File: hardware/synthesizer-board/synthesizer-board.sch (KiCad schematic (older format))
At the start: 193 parts, among them J1 SWD, J10 Conn_01x01, J11 Conn_01x01, J12 Conn_01x01, J13 Conn_01x01, J14 Conn_01x01, J15 Conn_01x01, J16 Conn_01x01, J17 Conn_01x01, J18 Conn_01x01, J19 Conn_01x01, J2 Conn_01x01, J20 Conn_01x01, J21 Conn_01x01, J22 Conn_01x01, J23 Conn_01x01, J3 Conn_01x01, J4 Conn_01x07, J5 Conn_01x01, J6 Conn_01x01, J7 Conn_01x01, J751 SELECTOR, J8 Conn_01x01, J9 Conn_01x01, P601 Conn_01x06_Male, P602 Conn_01x16_Male, P603 JST NH, P604 JST NH, Q101 BC847, Q201 BC847, Q301 BC847, Q401 BC847, Q701 BC847, Q702 BC847, Q703 BC847, Q704 BC847, Q705 BC847, Q721 BC847, Q731 BC847, Q741 BC847, Q751 BC847, Q811 BC847, Q821 BC847, Q831 BC847, Q841 BC847, Q851 BC847, Q861 BC847, Q871 BC847, U1 STM32G070RBTx, U101 U813, U11 LV2841XL, U21 LV2841XL, U601 LTV-247, U602 LTV-247, U603 LTV-247, U604 LTV-217, U605 AQY282SX, Y1 16MHz, Y2 32.768kHz

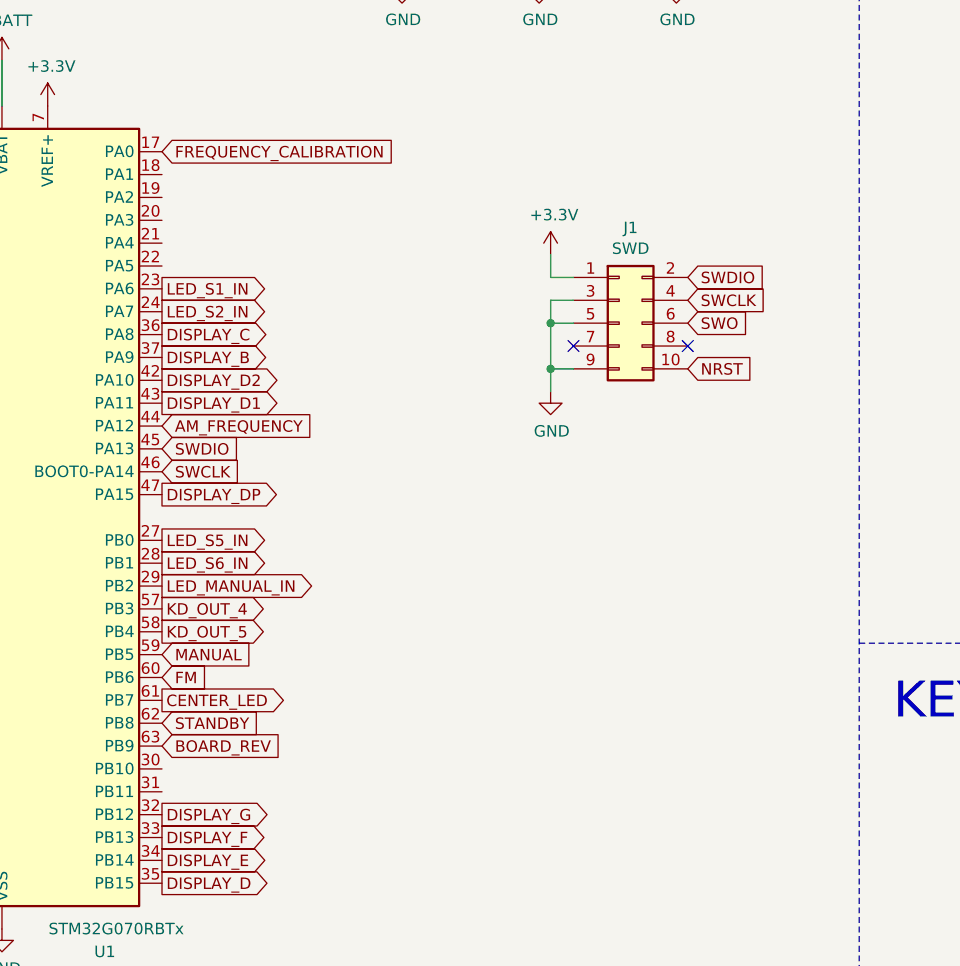
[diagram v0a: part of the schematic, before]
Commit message: Rev. C: Hardware
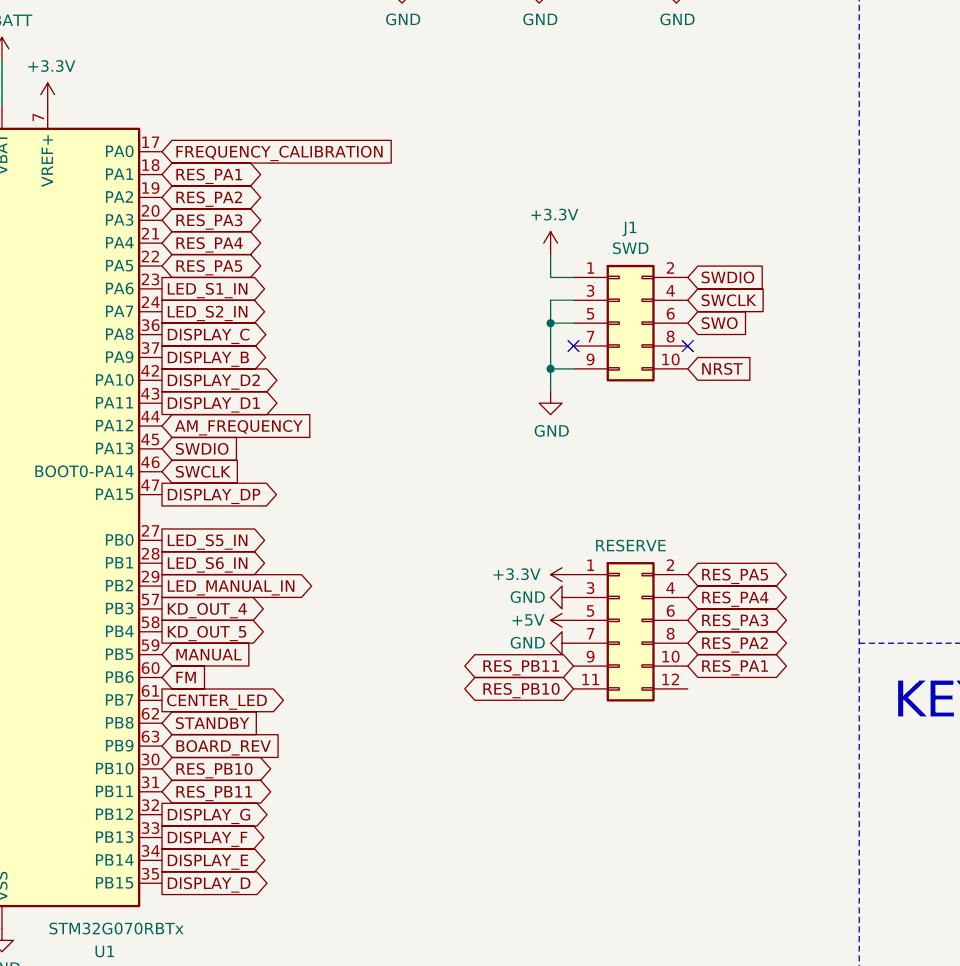
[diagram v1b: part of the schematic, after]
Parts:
- added J24: RESERVE, Pin_Headers:Pin_Header_Straight_2x06_Pitch2.54mm, symbol Connector_Generic:Conn_02x06_Odd_Even
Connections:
- net +3V3: now also J24.1 (Pin_1)
- net +5V: now also J24.5 (Pin_5)
- net GND: now also J24.3 (Pin_3), J24.7 (Pin_7)
- net RES_PA1: now reaches U1.18 (PA1)
- net RES_PA1: now also J24.10 (Pin_10)
- net RES_PA2: now reaches U1.19 (PA2)
- net RES_PA2: now also J24.8 (Pin_8)
- net RES_PA3: now reaches U1.20 (PA3)
- net RES_PA3: now also J24.6 (Pin_6)
- net RES_PA4: now reaches U1.21 (PA4)
- net RES_PA4: now also J24.4 (Pin_4)
- net RES_PA5: now reaches U1.22 (PA5)
- net RES_PA5: now also J24.2 (Pin_2)
- net RES_PB10: now reaches U1.30 (PB10)
- net RES_PB10: now also J24.11 (Pin_11)
- net RES_PB11: now reaches U1.31 (PB11)
- net RES_PB11: now also J24.9 (Pin_9)
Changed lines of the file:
@@
 	22400 13950 22250 13950
 Connection ~ 22250 13950
+Text GLabel 4950 2250 2    50   BiDi ~ 0
+RES_PA1
+Text GLabel 4950 2350 2    50   BiDi ~ 0
+RES_PA2
+Text GLabel 4950 2450 2    50   BiDi ~ 0
+RES_PA3
+Text GLabel 4950 2550 2    50   BiDi ~ 0
+RES_PA4
+Text GLabel 4950 2650 2    50   BiDi ~ 0
+RES_PA5
+Text GLabel 4950 4850 2    50   BiDi ~ 0
+RES_PB10
+Text GLabel 4950 4950 2    50   BiDi ~ 0
+RES_PB11
+$Comp
+L Connector_Generic:Conn_02x06_Odd_Even J24
+U 1 1 622574A8
+P 6950 4200
+F 0 "J24" V 7167 4196 50  0001 C CNN
+F 1 "RESERVE" H 7000 4525 50  0000 C CNN
+F 2 "Pin_Headers:Pin_Header_Straight_2x06_Pitch2.54mm" H 6950 4200 50  0001 C CNN
+F 3 "~" H 6950 4200 50  0001 C CNN
+	1    6950 4200
+	1    0    0    -1
+$EndComp
+Text GLabel 7250 4400 2    50   BiDi ~ 0
+RES_PA1
+Text GLabel 7250 4300 2    50   BiDi ~ 0
+RES_PA2
+Text GLabel 7250 4200 2    50   BiDi ~ 0
+RES_PA3
+Text GLabel 7250 4100 2    50   BiDi ~ 0
+RES_PA4
+Text GLabel 7250 4000 2    50   BiDi ~ 0
+RES_PA5
+Text GLabel 6750 4500 0    50   BiDi ~ 0
+RES_PB10
+Text GLabel 6750 4400 0    50   BiDi ~ 0
+RES_PB11
+$Comp
+L power:+3.3V #PWR0164
+U 1 1 622994F9
+P 6750 4000
+F 0 "#PWR0164" H 6750 3850 50  0001 C CNN
+F 1 "+3.3V" V 6750 4250 50  0000 C CNN
+F 2 "" H 6750 4000 50  0001 C CNN
+F 3 "" H 6750 4000 50  0001 C CNN
+	1    6750 4000
+	0    -1   -1   0
+$EndComp
+$Comp
+L power:GND #PWR0165
+U 1 1 6229AF13
+P 6750 4300
+F 0 "#PWR0165" H 6750 4050 50  0001 C CNN
+F 1 "GND" V 6750 4100 50  0000 C CNN
+F 2 "" H 6750 4300 50  0001 C CNN
+F 3 "" H 6750 4300 50  0001 C CNN
+	1    6750 4300
+	0    1    1    0
+$EndComp
+$Comp
+L power:+5V #PWR0166
+U 1 1 6229AF1D
+P 6750 4200
+F 0 "#PWR0166" H 6750 4050 50  0001 C CNN
+F 1 "+5V" V 6750 4400 50  0000 C CNN
+F 2 "" H 6750 4200 50  0001 C CNN
+F 3 "" H 6750 4200 50  0001 C CNN
+	1    6750 4200
+	0    -1   -1   0
+$EndComp
+$Comp
+L power:GND #PWR0167
+U 1 1 6229AF27
+P 6750 4100
+F 0 "#PWR0167" H 6750 3850 50  0001 C CNN
+F 1 "GND" V 6750 3900 50  0000 C CNN
+F 2 "" H 6750 4100 50  0001 C CNN
+F 3 "" H 6750 4100 50  0001 C CNN
+	1    6750 4100
+	0    1    1    0
+$EndComp
 $EndSCHEMATC
